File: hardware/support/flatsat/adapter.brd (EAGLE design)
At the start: 26 x 19 mm, 2 parts, among them X1 FH12-40S-0.5SH

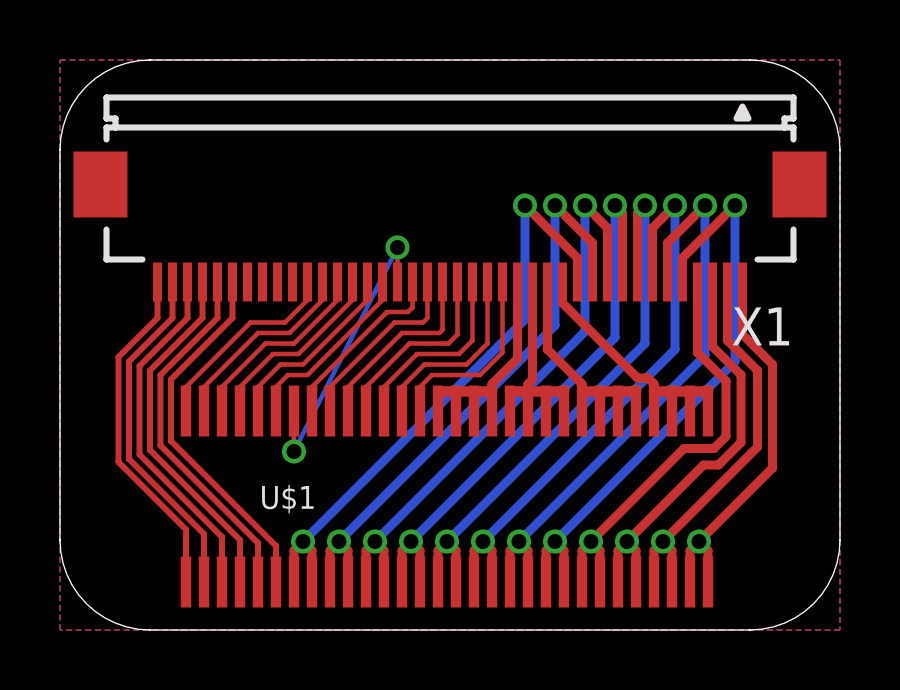
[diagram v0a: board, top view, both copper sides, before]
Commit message: merged master updates
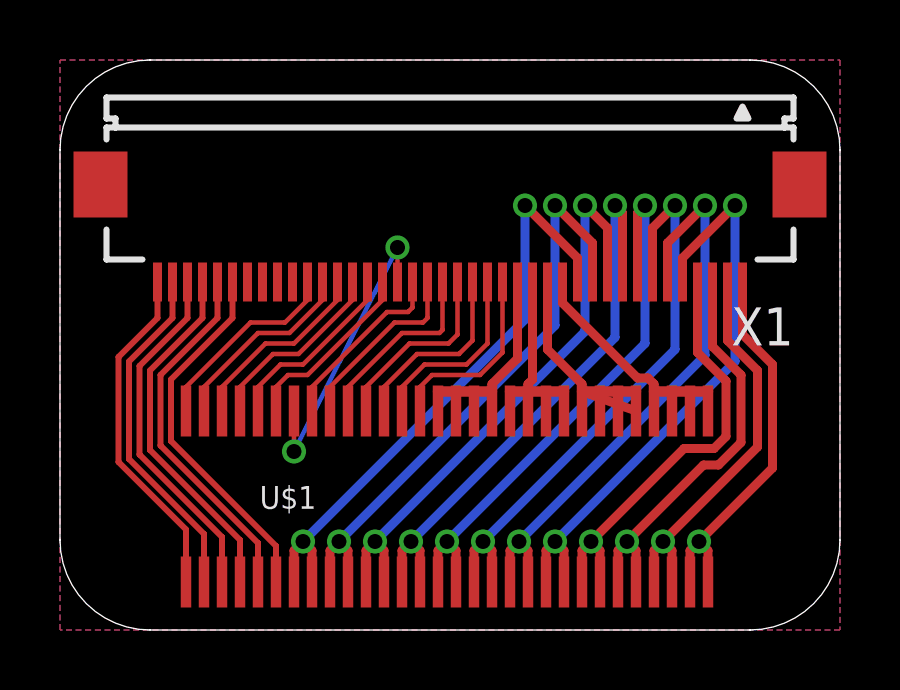
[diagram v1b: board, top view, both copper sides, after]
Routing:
- net RTN_+3V3: track 6.58 -> 7.84 mm
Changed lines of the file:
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@@
 </signal>
 <signal name="RTN_+3V3">
+<contactref element="U$1" pad="P$53"/>
+<contactref element="U$1" pad="P$54"/>
+<contactref element="U$1" pad="P$55"/>
 <contactref element="U$1" pad="P$56"/>
-<contactref element="U$1" pad="P$55"/>
-<contactref element="U$1" pad="P$54"/>
-<contactref element="U$1" pad="P$53"/>
 <contactref element="X1" pad="14"/>
 <wire x1="16.25" y1="11.6" x2="16.25" y2="9.35" width="0.3" layer="1"/>
 <wire x1="16.25" y1="9.35" x2="17.4" y2="8.2" width="0.3" layer="1"/>
 <wire x1="17.4" y1="8.2" x2="17.4" y2="7.95" width="0.3" layer="1"/>
-<wire x1="17.4" y1="7.95" x2="17.4" y2="7.3" width="0.3" layer="1"/>
+<wire x1="17.4" y1="7.95" x2="19.2" y2="7.3" width="0.3" layer="1"/>
 <wire x1="17.4" y1="7.95" x2="19.2" y2="7.95" width="0.35" layer="1"/>
 <wire x1="18.6" y1="7.3" x2="19.2" y2="7.3" width="0" layer="19" extent="1-1"/>
-<wire x1="18" y1="7.3" x2="18.6" y2="7.3" width="0" layer="19" extent="1-1"/>
-<wire x1="17.4" y1="7.3" x2="18" y2="7.3" width="0" layer="19" extent="1-1"/>
+<wire x1="18.6" y1="7.3" x2="18.6" y2="7.3" width="0" layer="19" extent="1-1"/>
+<wire x1="19.2" y1="7.3" x2="18.6" y2="7.3" width="0" layer="19" extent="1-1"/>
 </signal>
 <signal name="RTN_BATV">
+<contactref element="U$1" pad="P$45"/>
+<contactref element="U$1" pad="P$46"/>
+<contactref element="U$1" pad="P$47"/>
 <contactref element="U$1" pad="P$48"/>
-<contactref element="U$1" pad="P$47"/>
-<contactref element="U$1" pad="P$46"/>
-<contactref element="U$1" pad="P$45"/>
 <contactref element="X1" pad="16"/>
 <wire x1="15.25" y1="11.6" x2="15.25" y2="9.05" width="0.3" layer="1"/>
@@
 <wire x1="14.4" y1="7.95" x2="14.4" y2="7.3" width="0.3" layer="1"/>
 <wire x1="14.4" y1="7.95" x2="12.6" y2="7.95" width="0.35" layer="1"/>
-<wire x1="13.2" y1="7.3" x2="13.8" y2="7.3" width="0" layer="19" extent="1-1"/>
+<wire x1="13.8" y1="7.3" x2="13.8" y2="7.3" width="0" layer="19" extent="1-1"/>
 <wire x1="14.4" y1="7.3" x2="13.8" y2="7.3" width="0" layer="19" extent="1-1"/>
-<wire x1="12.6" y1="7.3" x2="13.2" y2="7.3" width="0" layer="19" extent="1-1"/>
+<wire x1="14.4" y1="7.3" x2="13.8" y2="7.3" width="0" layer="19" extent="1-1"/>
 </signal>
 <signal name="GPIO10">
@@
 </signal>
 <signal name="BATV_BUS">
+<contactref element="U$1" pad="P$52"/>
+<contactref element="U$1" pad="P$51"/>
+<contactref element="U$1" pad="P$50"/>
 <contactref element="U$1" pad="P$49"/>
-<contactref element="U$1" pad="P$50"/>
-<contactref element="U$1" pad="P$51"/>
-<contactref element="U$1" pad="P$52"/>
 <contactref element="X1" pad="15"/>
 <wire x1="15.75" y1="11.6" x2="15.75" y2="8.35" width="0.3" layer="1"/>
 <wire x1="15.75" y1="8.35" x2="15.6" y2="8.2" width="0.3" layer="1"/>
 <wire x1="15.6" y1="8.2" x2="15.6" y2="7.3" width="0.3" layer="1"/>
-<wire x1="16.8" y1="7.3" x2="16.2" y2="7.3" width="0" layer="19" extent="1-1"/>
-<wire x1="15.6" y1="7.3" x2="16.2" y2="7.3" width="0" layer="19" extent="1-1"/>
+<wire x1="15" y1="7.3" x2="15.6" y2="7.3" width="0" layer="19" extent="1-1"/>
+<wire x1="15.6" y1="7.3" x2="15.6" y2="7.3" width="0" layer="19" extent="1-1"/>
 <wire x1="15" y1="7.3" x2="15.6" y2="7.3" width="0" layer="19" extent="1-1"/>
 </signal>
@@
 </signal>
 <signal name="+3V3_BUS">
+<contactref element="U$1" pad="P$60"/>
+<contactref element="U$1" pad="P$59"/>
+<contactref element="U$1" pad="P$58"/>
 <contactref element="U$1" pad="P$57"/>
-<contactref element="U$1" pad="P$58"/>
-<contactref element="U$1" pad="P$59"/>
-<contactref element="U$1" pad="P$60"/>
 <contactref element="X1" pad="13"/>
 <wire x1="16.75" y1="11.6" x2="16.75" y2="10.9" width="0.3" layer="1"/>
@@
 <wire x1="19.8" y1="7.95" x2="19.8" y2="7.3" width="0.3" layer="1"/>
 <wire x1="19.8" y1="7.95" x2="21.6" y2="7.95" width="0.35" layer="1"/>
-<wire x1="21" y1="7.3" x2="20.4" y2="7.3" width="0" layer="19" extent="1-1"/>
-<wire x1="21.6" y1="7.3" x2="21" y2="7.3" width="0" layer="19" extent="1-1"/>
+<wire x1="20.4" y1="7.3" x2="20.4" y2="7.3" width="0" layer="19" extent="1-1"/>
+<wire x1="19.8" y1="7.3" x2="20.4" y2="7.3" width="0" layer="19" extent="1-1"/>
 <wire x1="19.8" y1="7.3" x2="20.4" y2="7.3" width="0" layer="19" extent="1-1"/>
 </signal>
